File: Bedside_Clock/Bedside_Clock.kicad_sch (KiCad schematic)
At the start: 35 parts, among them J1 USBC_USB2.0, SW1 COLOR, SW2 MODE, SW3 BOOT, SW4 RESET, U1 ESP32-C3-MINI-1, U2 USBLC6-2SC6

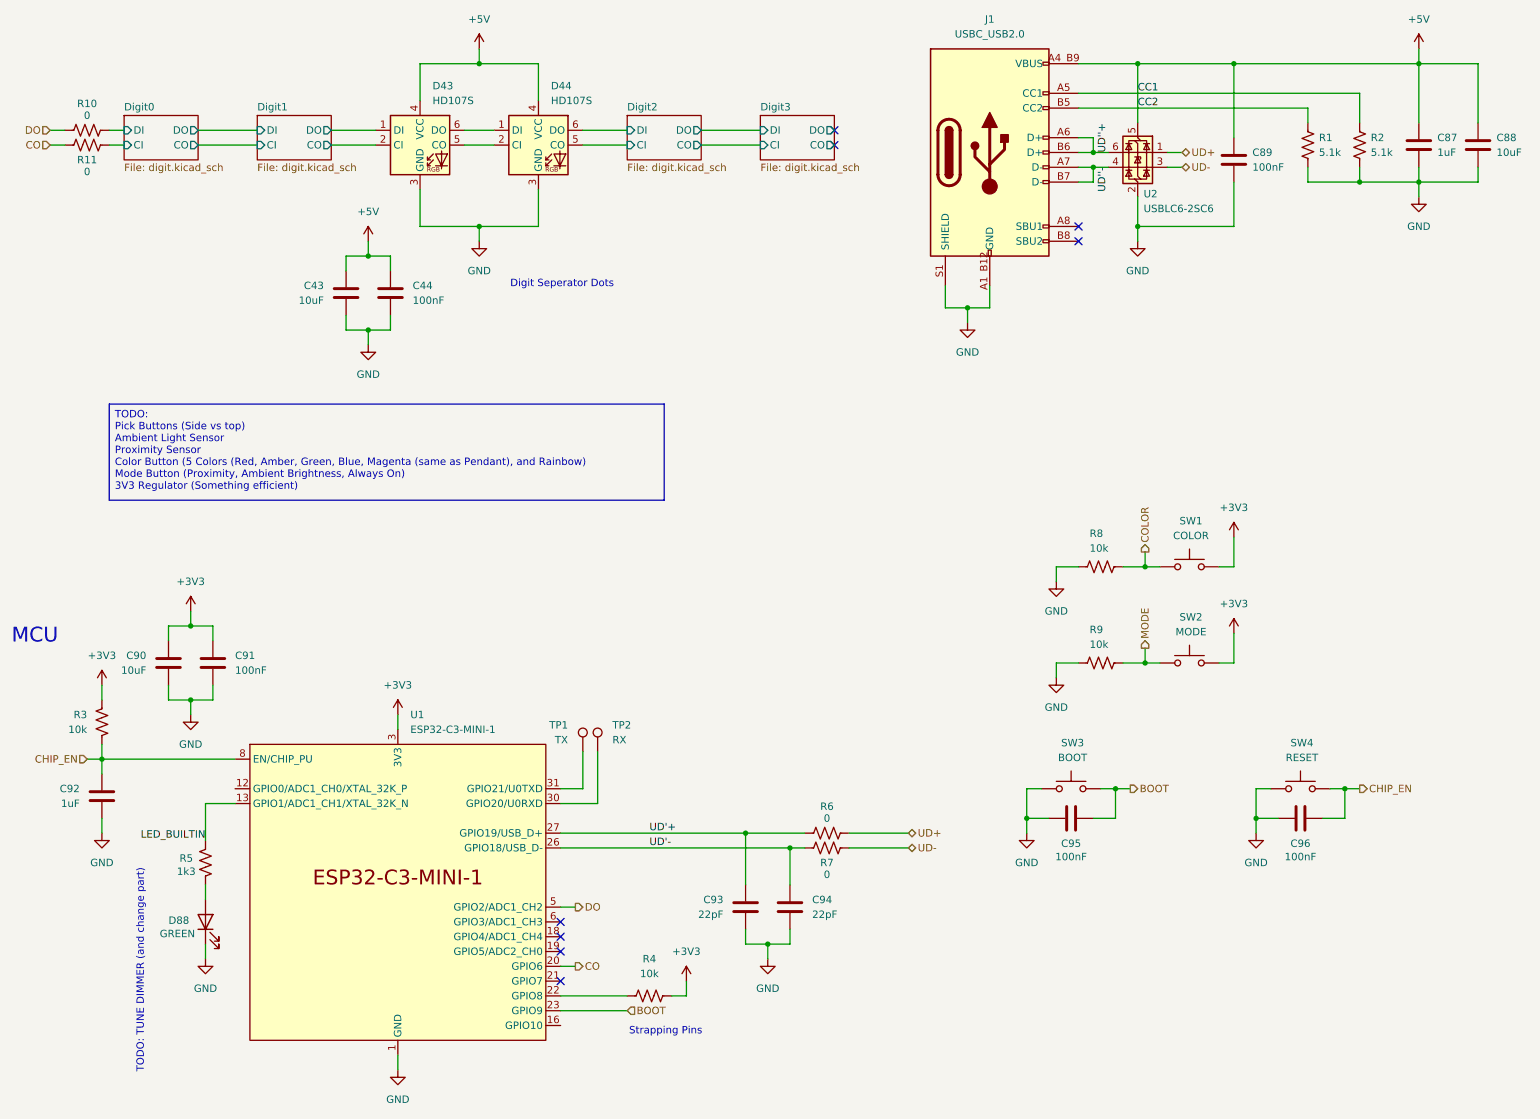
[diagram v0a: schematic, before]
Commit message: [HW] Clean up and layout improvements
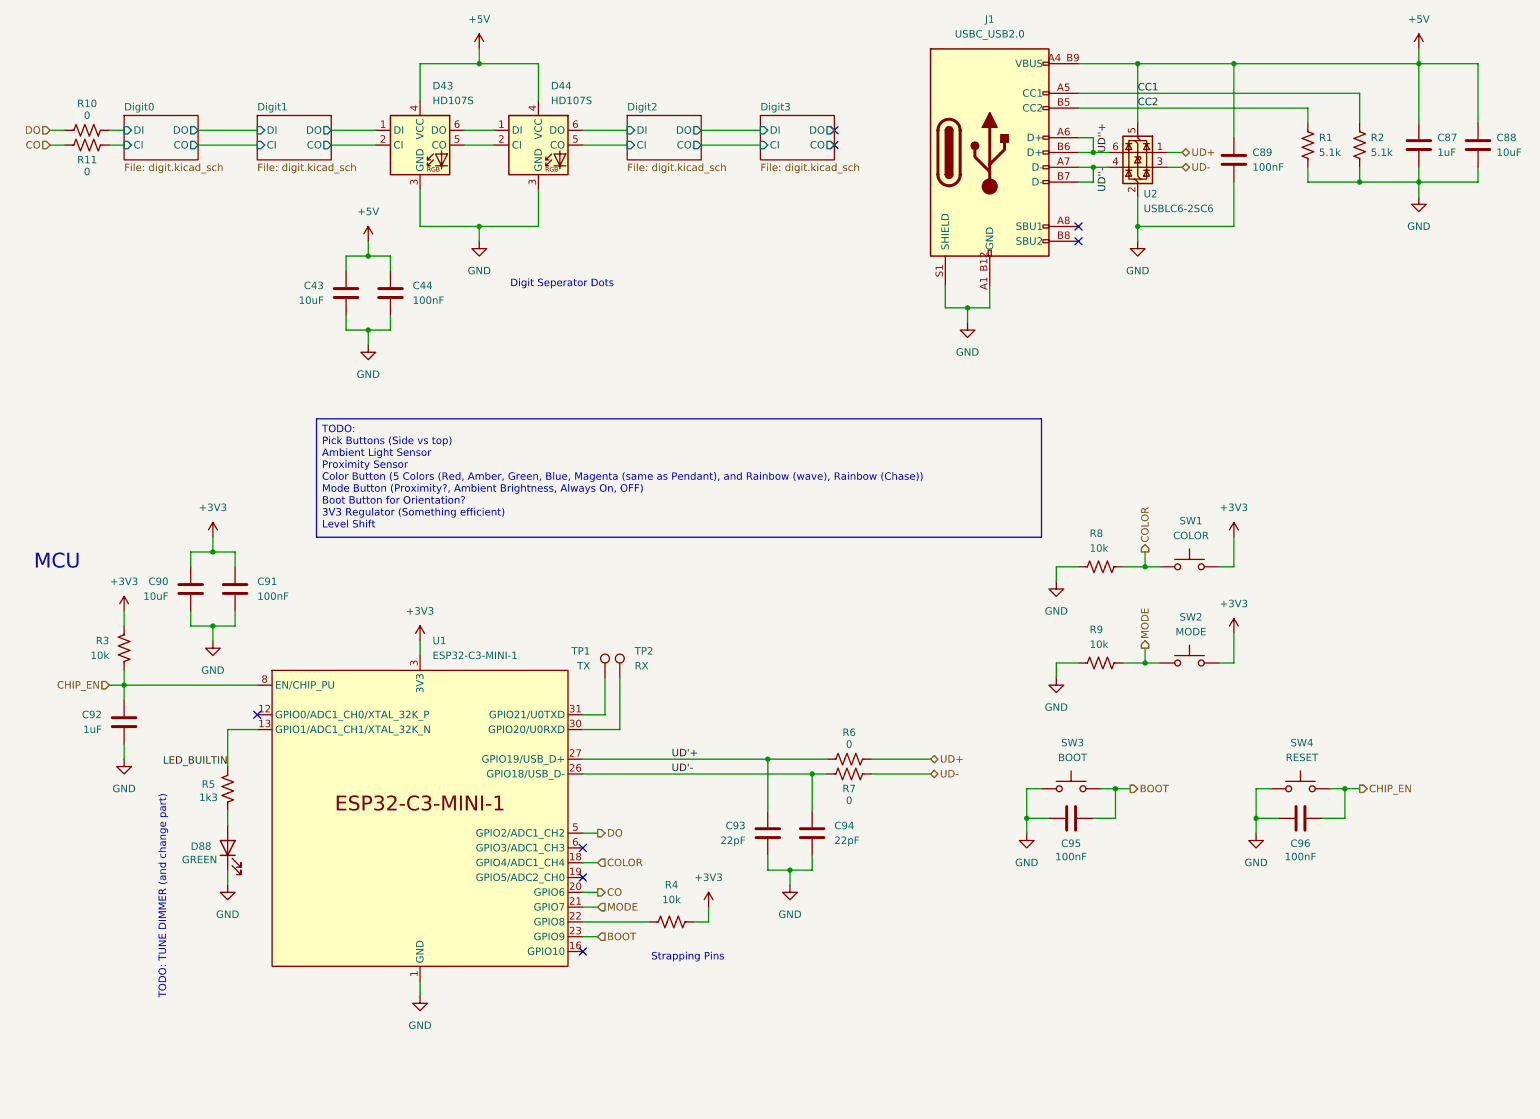
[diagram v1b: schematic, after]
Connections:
- net COLOR: now also U1.18 (GPIO4/ADC1_CH4)
- net MODE: now also U1.21 (GPIO7)
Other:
- moved on the sheet: C90, C91, C92, C93, C94, D88, R3, R4, R5, R6, R7, TP1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
